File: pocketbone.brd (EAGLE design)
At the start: 55 x 35 mm, 60 parts, among them J1 USD_CONNECTOR, U1 24LC_32AT-I/OT, U2 OSD3358, U3 SN74LVC1G07_DCK_5, Y1 CM200C-32.768KAZF-UT, Y2 445C33D24M00000

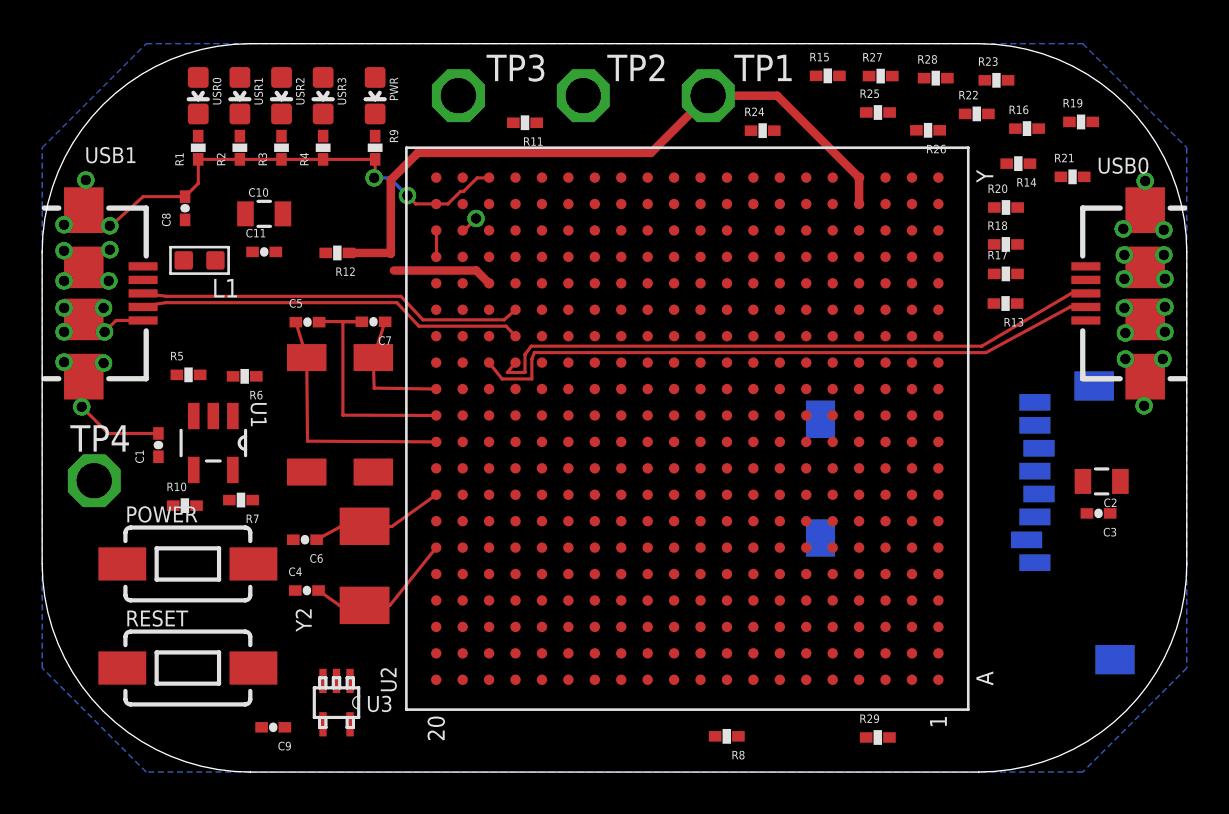
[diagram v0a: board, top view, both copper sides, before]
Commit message: Hack layout
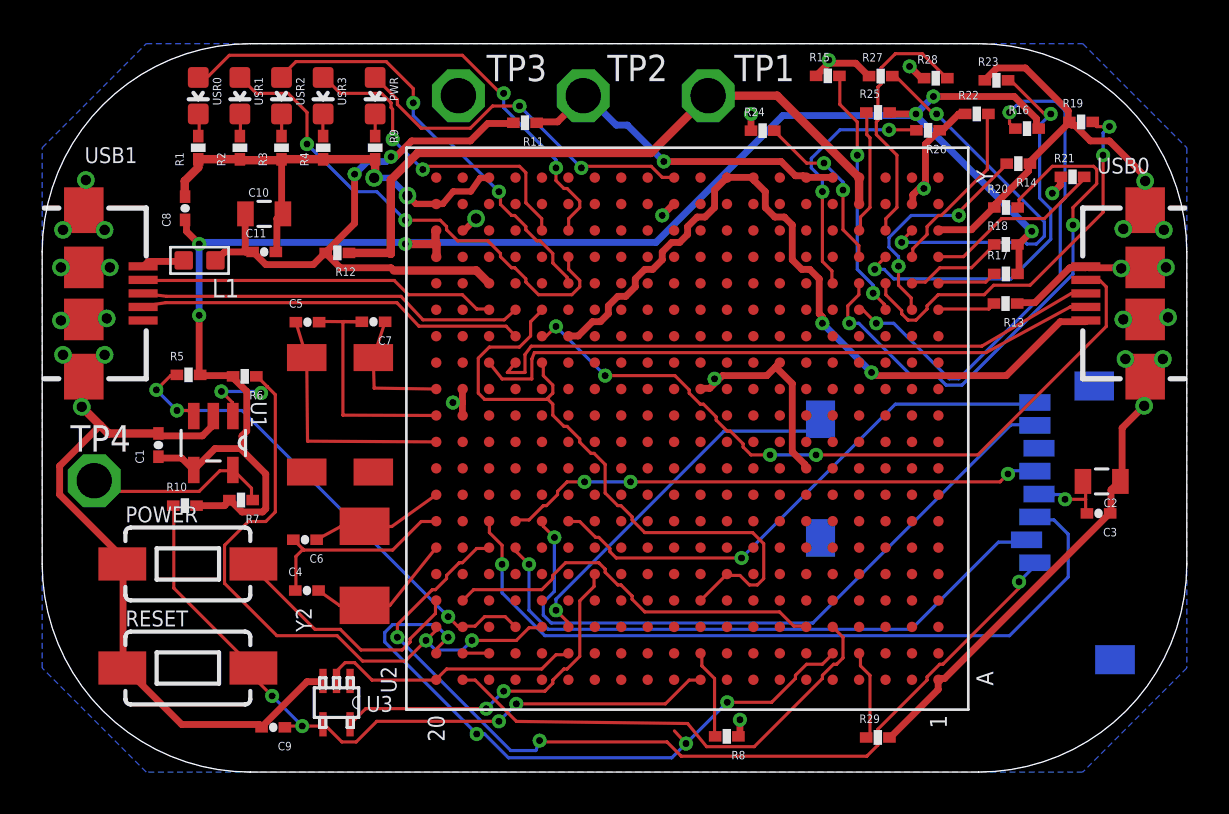
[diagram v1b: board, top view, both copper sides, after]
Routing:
- net GND: track 34.7 -> 135.1 mm, vias 31 -> 32
- net 3.3V: track 1.28 -> 83.6 mm, vias 0 -> 6
- net NTE: track 0.00 -> 44.9 mm, vias 0 -> 3
- net USB_DC: track 0.00 -> 37.1 mm, vias 0 -> 2
- net N$74: track 0.00 -> 37.0 mm, vias 0 -> 1
- net USB0_ID: track 0.00 -> 35.7 mm, vias 0 -> 4
- net RESET: track 0.00 -> 34.9 mm, vias 0 -> 4
- net I2C0_SCL: track 0.00 -> 34.3 mm, vias 0 -> 4
- net N$77: track 0.00 -> 32.7 mm, vias 0 -> 1
- net VDD_1V8: track 0.00 -> 31.8 mm
- net LDO_PGOOD: track 0.00 -> 31.8 mm, vias 0 -> 4
- net N$5: track 0.00 -> 29.3 mm, vias 0 -> 1
- net SVO6: track 0.00 -> 26.7 mm, vias 0 -> 2
- net N$70: track 0.00 -> 26.3 mm, vias 0 -> 1
- net N$2: track 0.00 -> 26.1 mm, vias 0 -> 3
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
